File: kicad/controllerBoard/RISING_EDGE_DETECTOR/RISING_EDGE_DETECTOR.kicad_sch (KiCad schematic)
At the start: 14 parts, among them Q385 PMOS, Q386 NMOS, Q391 PMOS, Q392 NMOS, Q393 PMOS, Q394 NMOS, Q425 PMOS, Q426 NMOS

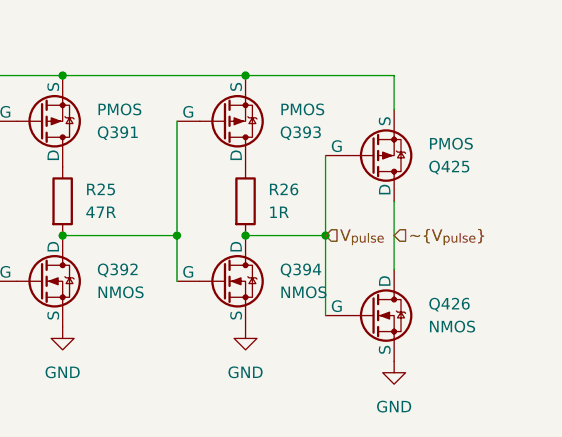
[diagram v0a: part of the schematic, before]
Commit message: stuff
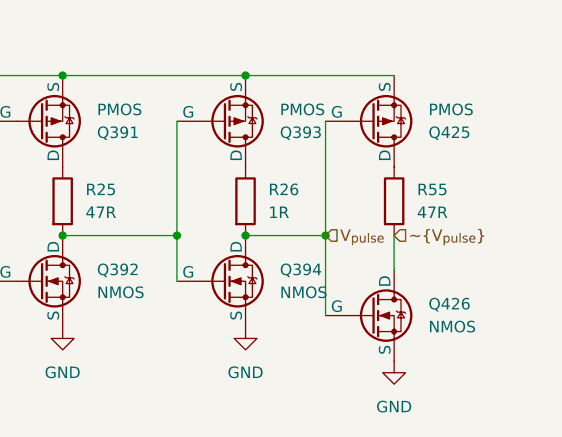
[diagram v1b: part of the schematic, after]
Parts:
- added R55: 47R, symbol Device:R
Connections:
- net ~{V_{pulse}}: now also R55.2; no longer Q425.1 (D)
- new net: Q425.1 (D), R55.1
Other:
- moved on the sheet: Q425
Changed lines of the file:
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@@
+	)
+	(junction
+		(at 166.37 66.04)
+		(diameter 0)
+		(color 0 0 0 0)
 	)
 	(junction
@@
 	)
 	(junction
-		(at 166.37 66.04)
-		(diameter 0)
-		(color 0 0 0 0)
-	)
-	(junction
 		(at 157.48 66.04)
 		(diameter 0)
@@
 	(wire
 		(pts
-			(xy 166.37 57.15) (xy 166.37 66.04)
+			(xy 166.37 53.34) (xy 166.37 66.04)
 		)
 		(stroke
@@
 	(wire
 		(pts
-			(xy 81.28 53.34) (xy 81.28 66.04)
+			(xy 173.99 66.04) (xy 173.99 69.85)
 		)
 		(stroke
@@
 	(wire
 		(pts
-			(xy 111.76 66.04) (xy 120.65 66.04)
+			(xy 81.28 53.34) (xy 81.28 66.04)
 		)
 		(stroke
@@
 	(wire
 		(pts
-			(xy 166.37 66.04) (xy 166.37 74.93)
+			(xy 111.76 66.04) (xy 120.65 66.04)
 		)
 		(stroke
@@
 	(wire
 		(pts
-			(xy 173.99 52.07) (xy 173.99 48.26)
-		)
-		(stroke
-			(width 0)
-			(type default)
-		)
-	)
-	(wire
-		(pts
-			(xy 173.99 62.23) (xy 173.99 69.85)
+			(xy 166.37 66.04) (xy 166.37 74.93)
 		)
 		(stroke
@@
 	(symbol
 		(lib_id "Simulation_SPICE:PMOS")
-		(at 171.45 57.15 0)
+		(at 171.45 53.34 0)
 		(mirror x)
 		(unit 1)
@@
 		(dnp no)
 		(property "Reference" "Q425"
-			(at 177.8 58.4201 0)
+			(at 177.8 54.6101 0)
 			(show_name no)
 			(do_not_autoplace no)
@@
 		)
 		(property "Value" "PMOS"
-			(at 177.8 55.8801 0)
+			(at 177.8 52.0701 0)
 			(show_name no)
 			(do_not_autoplace no)
@@
 		)
 		(property "Footprint" ""
-			(at 176.53 59.69 0)
+			(at 176.53 55.88 0)
 			(hide yes)
 			(show_name no)
@@
 		)
 		(property "Datasheet" "https://ngspice.sourceforge.io/docs/ngspice-html-manual/manual.xhtml#cha_MOSFETs"
-			(at 171.45 44.45 0)
+			(at 171.45 40.64 0)
 			(hide yes)
 			(show_name no)
@@
 		)
 		(property "Description" "P-MOSFET transistor, drain/source/gate"
-			(at 171.45 57.15 0)
+			(at 171.45 53.34 0)
 			(hide yes)
 			(show_name no)
@@
 		)
 		(property "Sim.Device" "PMOS"
-			(at 171.45 40.005 0)
+			(at 171.45 36.195 0)
 			(hide yes)
 			(show_name no)
@@
 		)
 		(property "Sim.Type" "VDMOS"
+			(at 171.45 34.29 0)
+			(hide yes)
+			(show_name no)
+			(do_not_autoplace no)
+			(effects
+				(font
+					(size 1.27 1.27)
+				)
+			)
+		)
+		(property "Sim.Pins" "1=D 2=G 3=S"
 			(at 171.45 38.1 0)
-			(hide yes)
-			(show_name no)
-			(do_not_autoplace no)
-			(effects
-				(font
-					(size 1.27 1.27)
-				)
-			)
-		)
-		(property "Sim.Pins" "1=D 2=G 3=S"
-			(at 171.45 41.91 0)
 			(hide yes)
 			(show_name no)
@@
 					(unit 1)
 				)
+			)
+		)
+	)
+	(symbol
+		(lib_id "Device:R")
+		(at 173.99 62.23 0)
+		(unit 1)
+		(body_style 1)
+		(exclude_from_sim no)
+		(in_bom yes)
+		(on_board yes)
+		(in_pos_files yes)
+		(dnp no)
+		(fields_autoplaced yes)
+		(property "Reference" "R55"
+			(at 176.53 60.9599 0)
+			(show_name no)
+			(do_not_autoplace no)
+			(effects
+				(font
+					(size 1.27 1.27)
+				)
+				(justify left)
+			)
+		)
+		(property "Value" "47R"
+			(at 176.53 63.4999 0)
+			(show_name no)
+			(do_not_autoplace no)
+			(effects
+				(font
+					(size 1.27 1.27)
+				)
+				(justify left)
+			)
+		)
+		(property "Footprint" ""
+			(at 172.212 62.23 90)
+			(hide yes)
+			(show_name no)
+			(do_not_autoplace no)
+			(effects
+				(font
+					(size 1.27 1.27)
+				)
+			)
+		)
+		(property "Datasheet" ""
+			(at 173.99 62.23 0)
+			(hide yes)
+			(show_name no)
+			(do_not_autoplace no)
+			(effects
+				(font
+					(size 1.27 1.27)
+				)
+			)
+		)
+		(property "Description" "Resistor"
+			(at 173.99 62.23 0)
+			(hide yes)
+			(show_name no)
+			(do_not_autoplace no)
+			(effects
+				(font
+					(size 1.27 1.27)
+				)
+			)
+		)
+		(pin "2"
+		)
+		(pin "1"
+		)
+		(instances
+			(project "controllerBoard"
+				(path "/93a9a1ca-4ee5-40da-ab67-92836146c003/96d1d3a9-3ebd-46ac-a2d2-b692fac1af2c"
+					(reference "R55")
+					(unit 1)
+				)
+				(path "/93a9a1ca-4ee5-40da-ab67-92836146c003/def1fdf8-7002-45c6-87e0-28926b899265"
+					(reference "R56")
+					(unit 1)
+				)
